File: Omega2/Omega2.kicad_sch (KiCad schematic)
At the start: 15 parts, among them J1 Conn_01x04_Female, J2 Conn_01x14_Female, J3 Conn_01x07_Female, SW1 SW_DIP_x01, SW2 FW, SW3 BW, U1 Omega2+

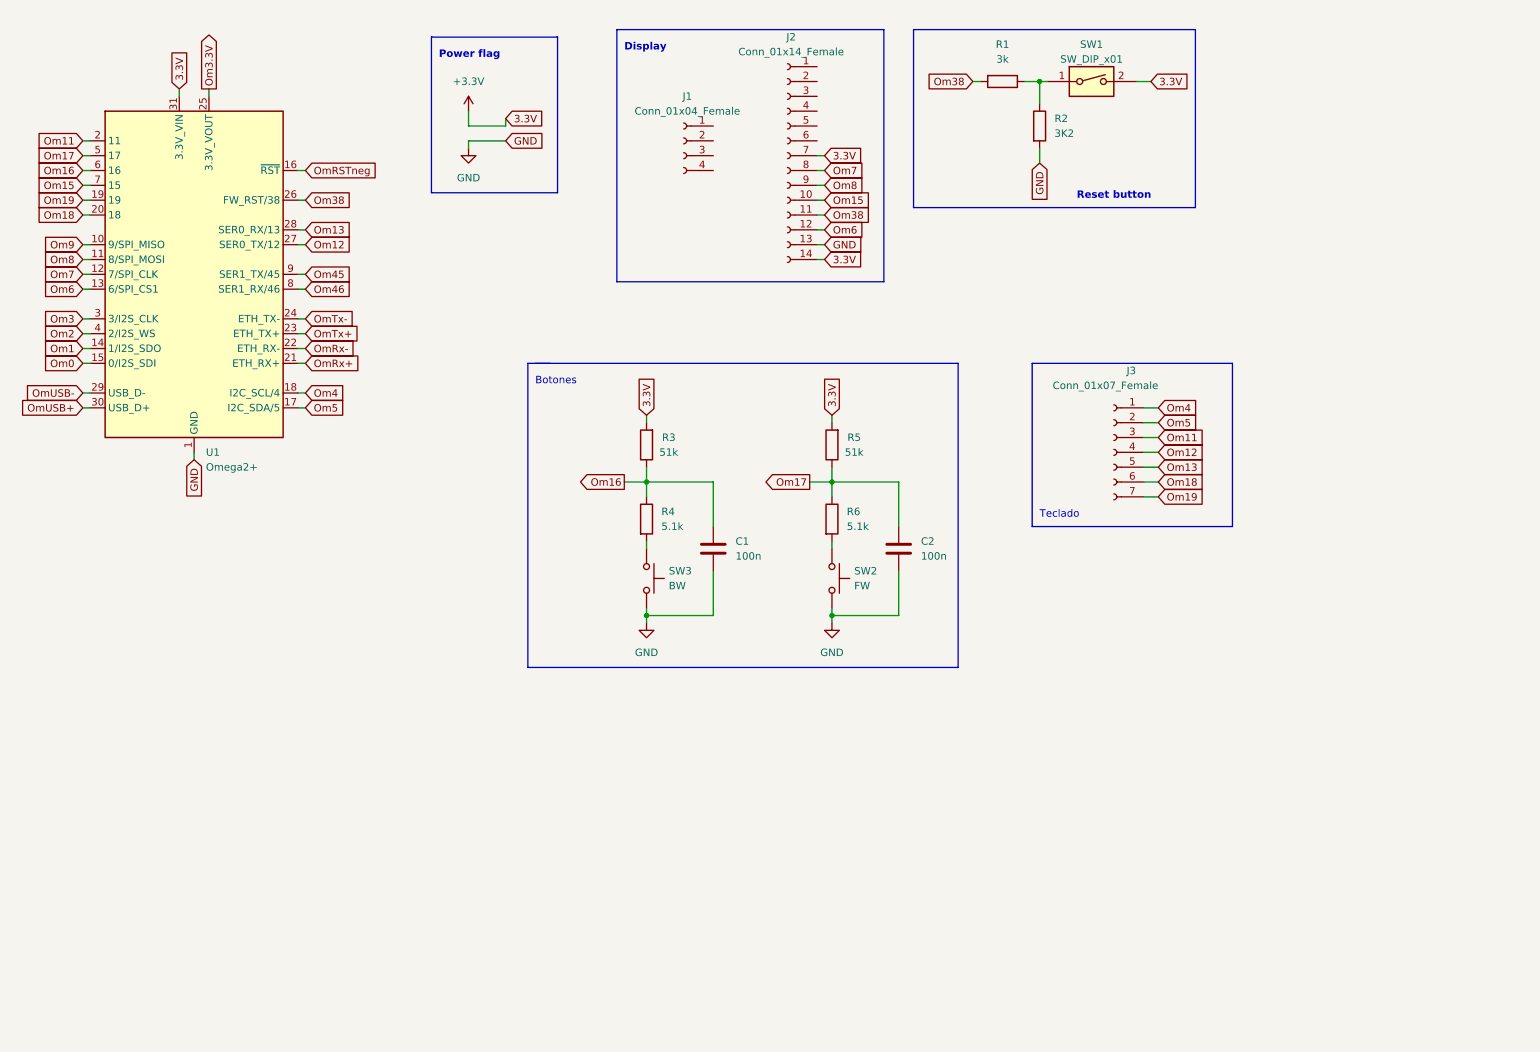
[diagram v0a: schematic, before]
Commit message: union de todo en el mismo esquemático
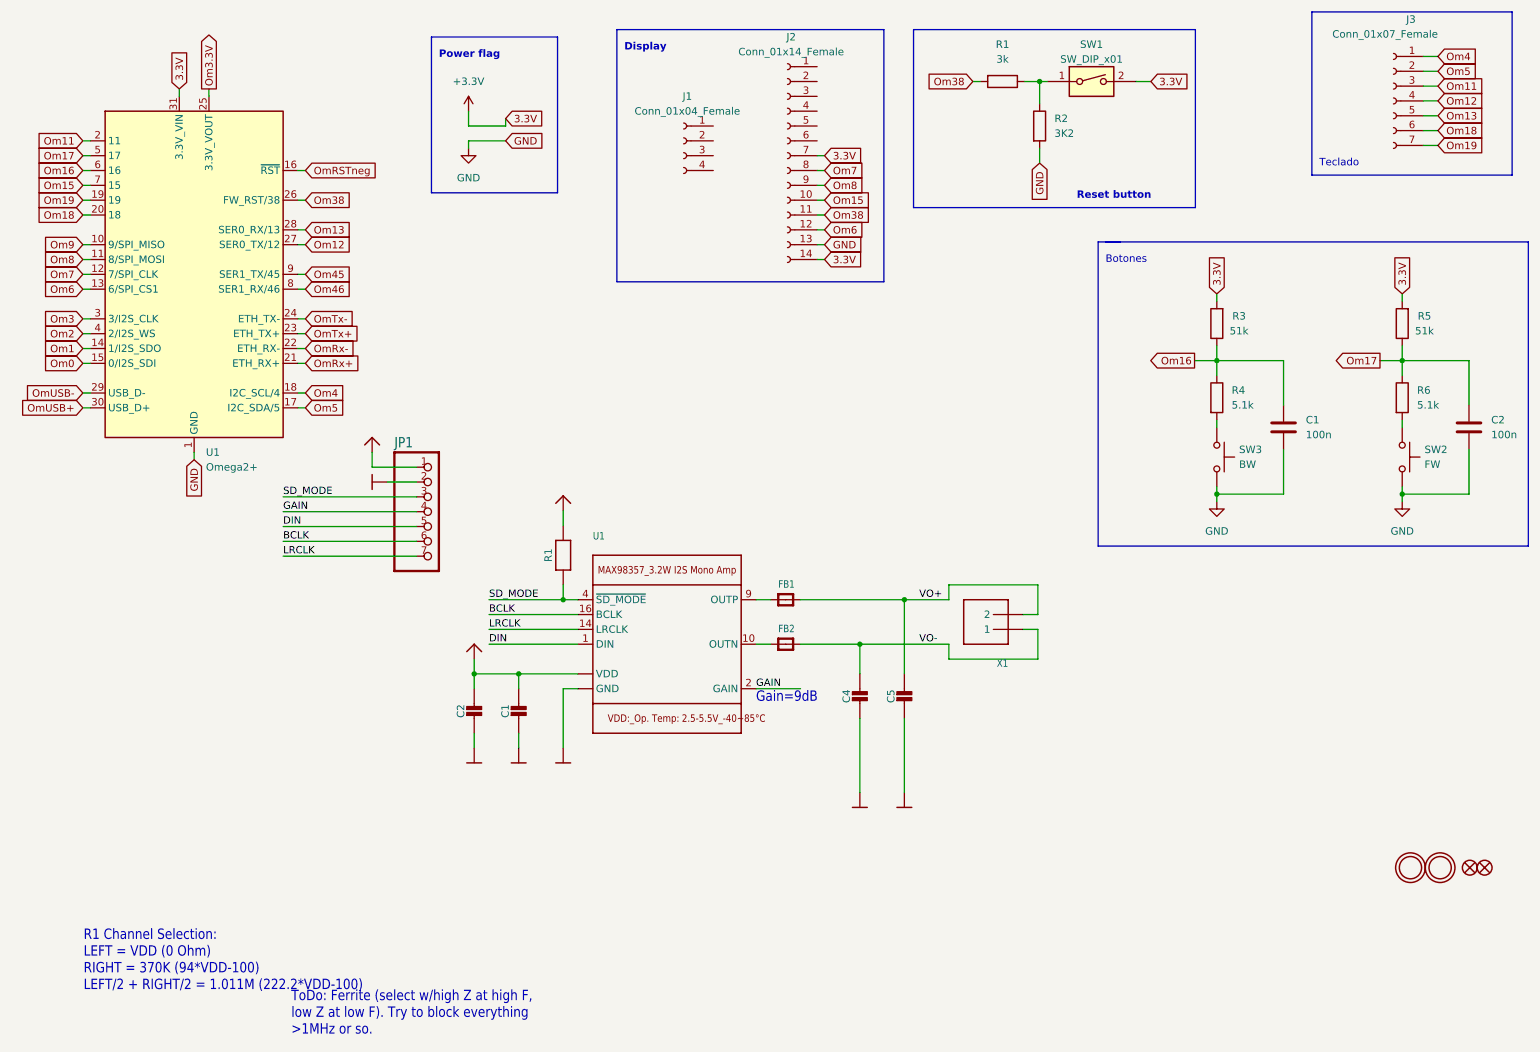
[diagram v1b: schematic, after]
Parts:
- added C1, C2, C4, C5: (no value), symbol Adafruit MAX98357 Breakout-eagle-import:CAP_CERAMIC0805-NOOUTLINE
- added FB1, FB2: (no value), symbol Adafruit MAX98357 Breakout-eagle-import:FERRITE-0805NO
- added FID1, FID2: (no value), symbol Adafruit MAX98357 Breakout-eagle-import:FIDUCIAL{dblquote}{dblquote}
- added JP1: (no value), symbol Adafruit MAX98357 Breakout-eagle-import:HEADER-1X7THICKER
- added R1: (no value), symbol Adafruit MAX98357 Breakout-eagle-import:RESISTOR0805_NOOUTLINE
- added U$10, U$9: (no value), symbol Adafruit MAX98357 Breakout-eagle-import:MOUNTINGHOLE2.5
- added U1: (no value), symbol Adafruit MAX98357 Breakout-eagle-import:AUDIOAMP_MAX98357
- added X1: (no value), symbol Adafruit MAX98357 Breakout-eagle-import:TERMBLOCK_1X2
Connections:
- net GND: now also C1.2, C2.2, C4.2, C5.2, JP1.2, U1.11 (GND), U1.15 (GND), U1.3 (GND), U1.THERMAL (GND)
- new net: FB1.1 (P$1), U1.9 (OUTP)
- new net: FB2.1 (P$1), U1.10 (OUTN)
- new net BCLK: JP1.6, U1.16 (BCLK)
- new net DIN: JP1.5, U1.1 (DIN)
- new net GAIN: JP1.4, U1.2 (GAIN)
- new net LRCLK: JP1.7, U1.14 (LRCLK)
- new net SD_MODE: JP1.3, R1.1, U1.4 (~{SD_MODE})
- new net VDD: C1.1, C2.1, JP1.1, R1.2, U1.7 (VDD), U1.8 (VDD)
- new net VO+: C5.1, FB1.2 (P$2), X1.2
- new net VO-: C4.1, FB2.2 (P$2), X1.1
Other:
- note added: "Gain=9dB"
- note added: "R1 Channel Selection: LEFT = VDD (0 Ohm) RIGHT = 370K (94*VDD-100) LEFT/2 + RIGHT/2 = 1.011M (222.2*VDD-100)"
- note added: "ToDo: Ferrite (select w/high Z at high F, low Z at low F). Try to block everything >1MHz or so."
- moved on the sheet: C1, C2, J3, R3, R4, R5, R6, SW2, SW3
